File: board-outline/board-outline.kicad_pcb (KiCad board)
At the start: 2 copper layers, 120 x 136.8 mm, 1 part

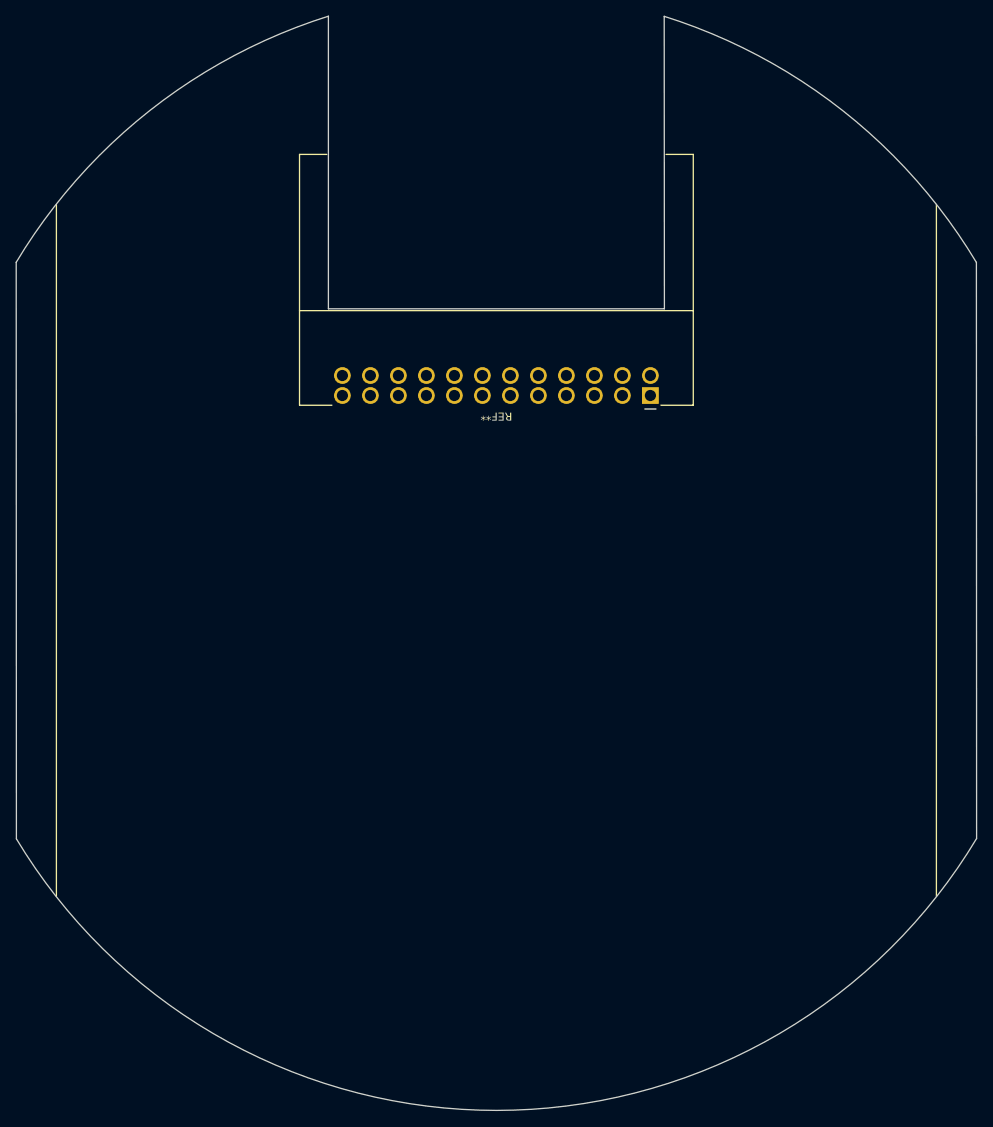
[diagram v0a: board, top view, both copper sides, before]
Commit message: New standard board
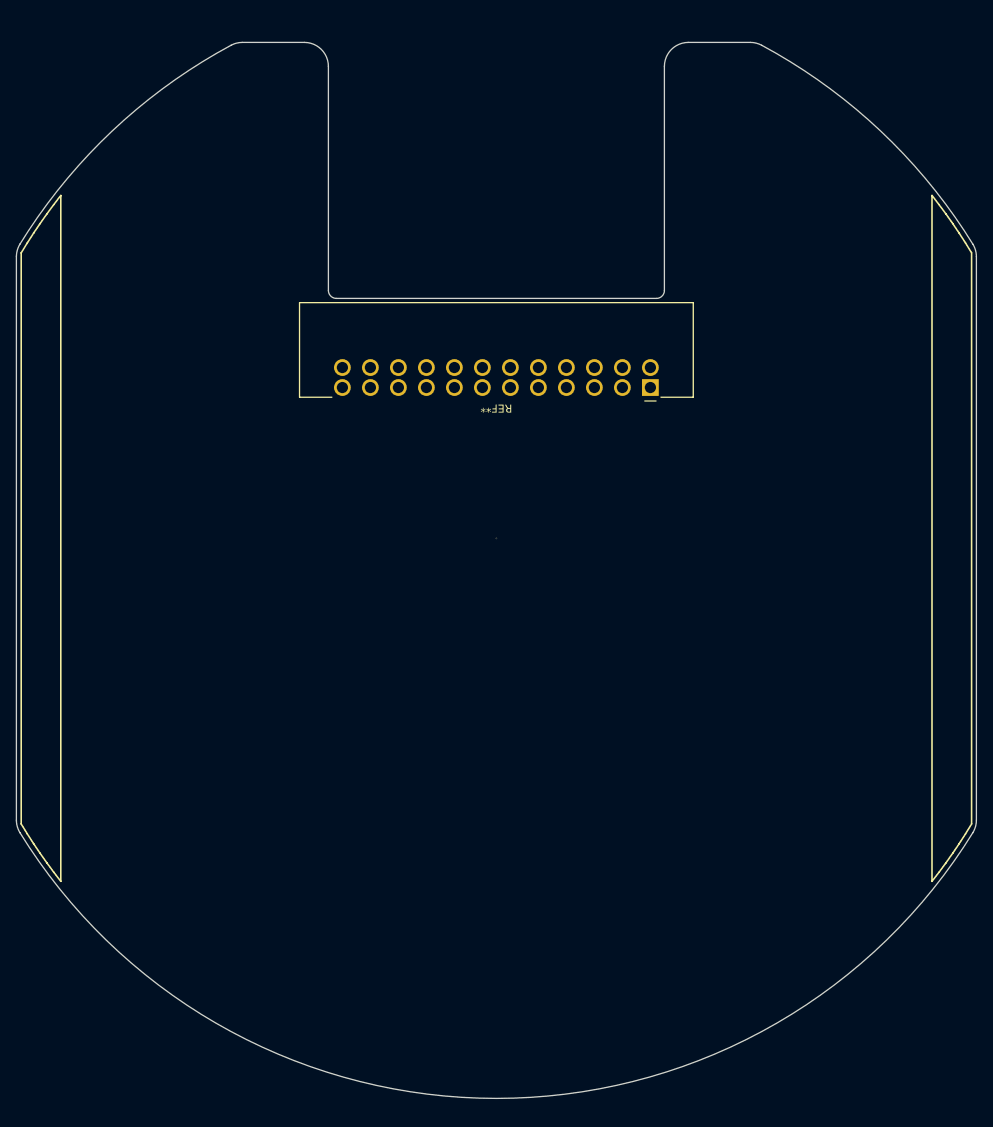
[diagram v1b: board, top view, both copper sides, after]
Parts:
- moved REF** 1.00 mm to (239.2, 108.6)
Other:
- board size 120 x 136.8 mm -> 120 x 132 mm

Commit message: Fixa board outkube
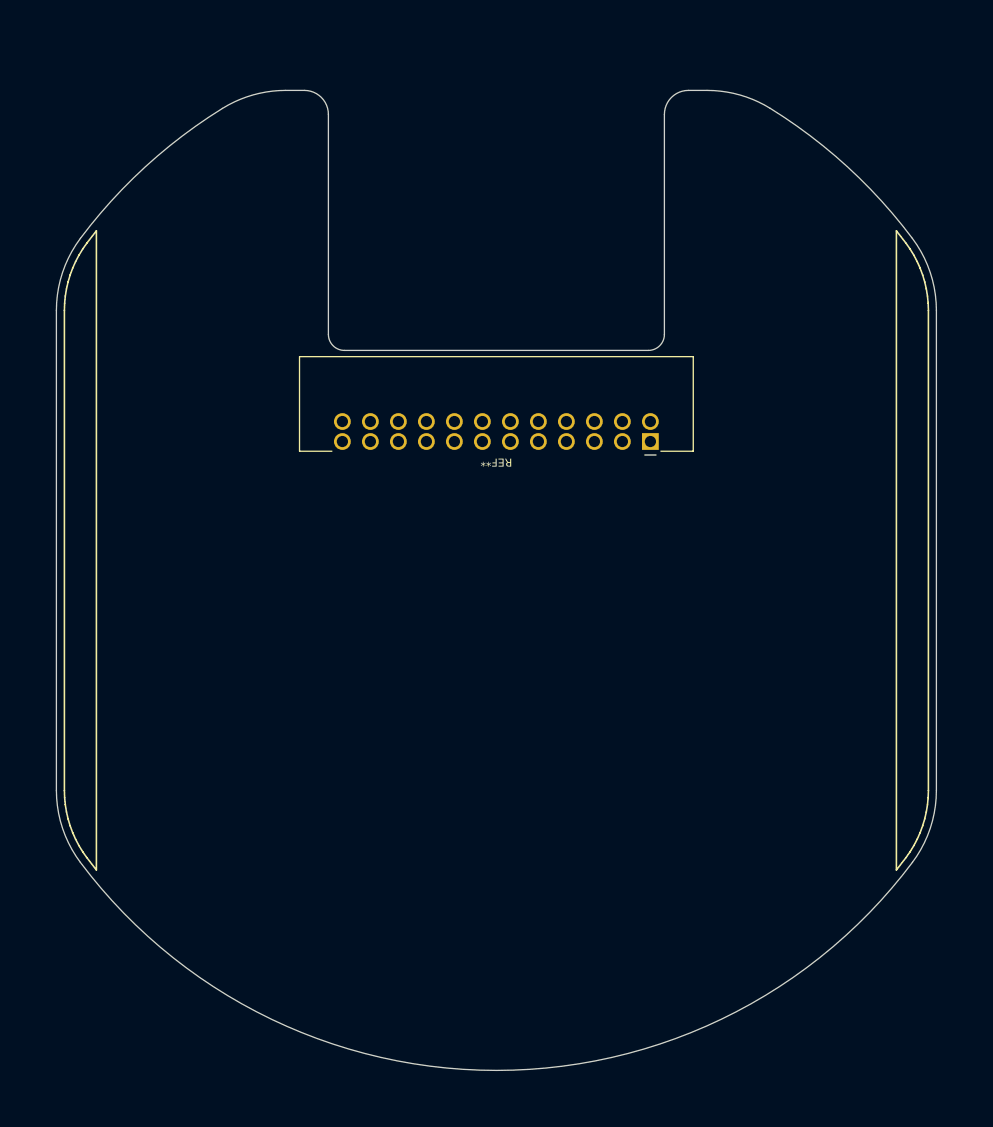
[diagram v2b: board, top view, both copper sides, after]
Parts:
- moved REF** 6.75 mm to (239.2, 115.4)
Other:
- board size 120 x 132 mm -> 110 x 122.5 mm
